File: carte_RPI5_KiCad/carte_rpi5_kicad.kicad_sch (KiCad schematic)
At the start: 0 parts

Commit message: Placement composants
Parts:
- added PS1: OKL-T_6-W12N-C, OKLT6W12NC, symbol Librairie_symbole:OKL-T_6-W12N-C
- added U1: CM5108032, CM5108032:MODULE_CM5108032, symbol Librairie_symbole:CM5108032
- added U2: BNO055, BNO055:LGA28R50P4X10_380X520X100, symbol Librairie_symbole:BNO055
- added U3: L293D, L293D:DIP880W50P254L2000H510Q16, symbol Librairie_symbole:L293D
- added U4: LPS22HB, LPS22HB:LGA10R50P2X3_200X200X80, symbol Librairie_symbole:LPS22HB
- added U5: PCA9685PW_118, PCA9685PW_118:SOP65P640X110-28N, symbol Librairie_symbole:PCA9685PW_118
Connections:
- new net: U1.SH1 (MOUNTING_PADS), U1.SH2 (MOUNTING_PADS), U1.SH3 (MOUNTING_PADS), U1.SH4 (MOUNTING_PADS)
- new net +5V(INPUT): U1.77 (+5V(INPUT)), U1.79 (+5V(INPUT)), U1.81 (+5V(INPUT)), U1.83 (+5V(INPUT)), U1.85 (+5V(INPUT)), U1.87 (+5V(INPUT))
- new net CM5_1.8V(OUTPUT): U1.88 (CM5_1.8V(OUTPUT)), U1.90 (CM5_1.8V(OUTPUT))
- new net CM5_3.3V(OUTPUT): U1.84 (CM5_3.3V(OUTPUT)), U1.86 (CM5_3.3V(OUTPUT))
- new net GND: U1.1 (GND), U1.107 (GND), U1.108 (GND), U1.113 (GND), U1.114 (GND), U1.119 (GND), U1.120 (GND), U1.125 (GND), U1.126 (GND), U1.13 (GND), U1.131 (GND), U1.132 (GND), U1.137 (GND), U1.138 (GND), U1.14 (GND), U1.144 (GND), U1.150 (GND), U1.155 (GND), U1.156 (GND), U1.161 (GND), U1.162 (GND), U1.167 (GND), U1.168 (GND), U1.173 (GND), U1.174 (GND), U1.179 (GND), U1.180 (GND), U1.185 (GND), U1.186 (GND), U1.191 (GND), U1.192 (GND), U1.197 (GND), U1.198 (GND), U1.2 (GND), U1.22 (GND), U1.23 (GND), U1.32 (GND), U1.33 (GND), U1.42 (GND), U1.43 (GND), U1.52 (GND), U1.53 (GND), U1.59 (GND), U1.60 (GND), U1.65 (GND), U1.66 (GND), U1.7 (GND), U1.71 (GND), U1.74 (GND), U1.8 (GND), U1.98 (GND), U3.12 (GND), U3.13 (GND), U3.4 (GND), U3.5 (GND), U4.8 (GND), U4.9 (GND)

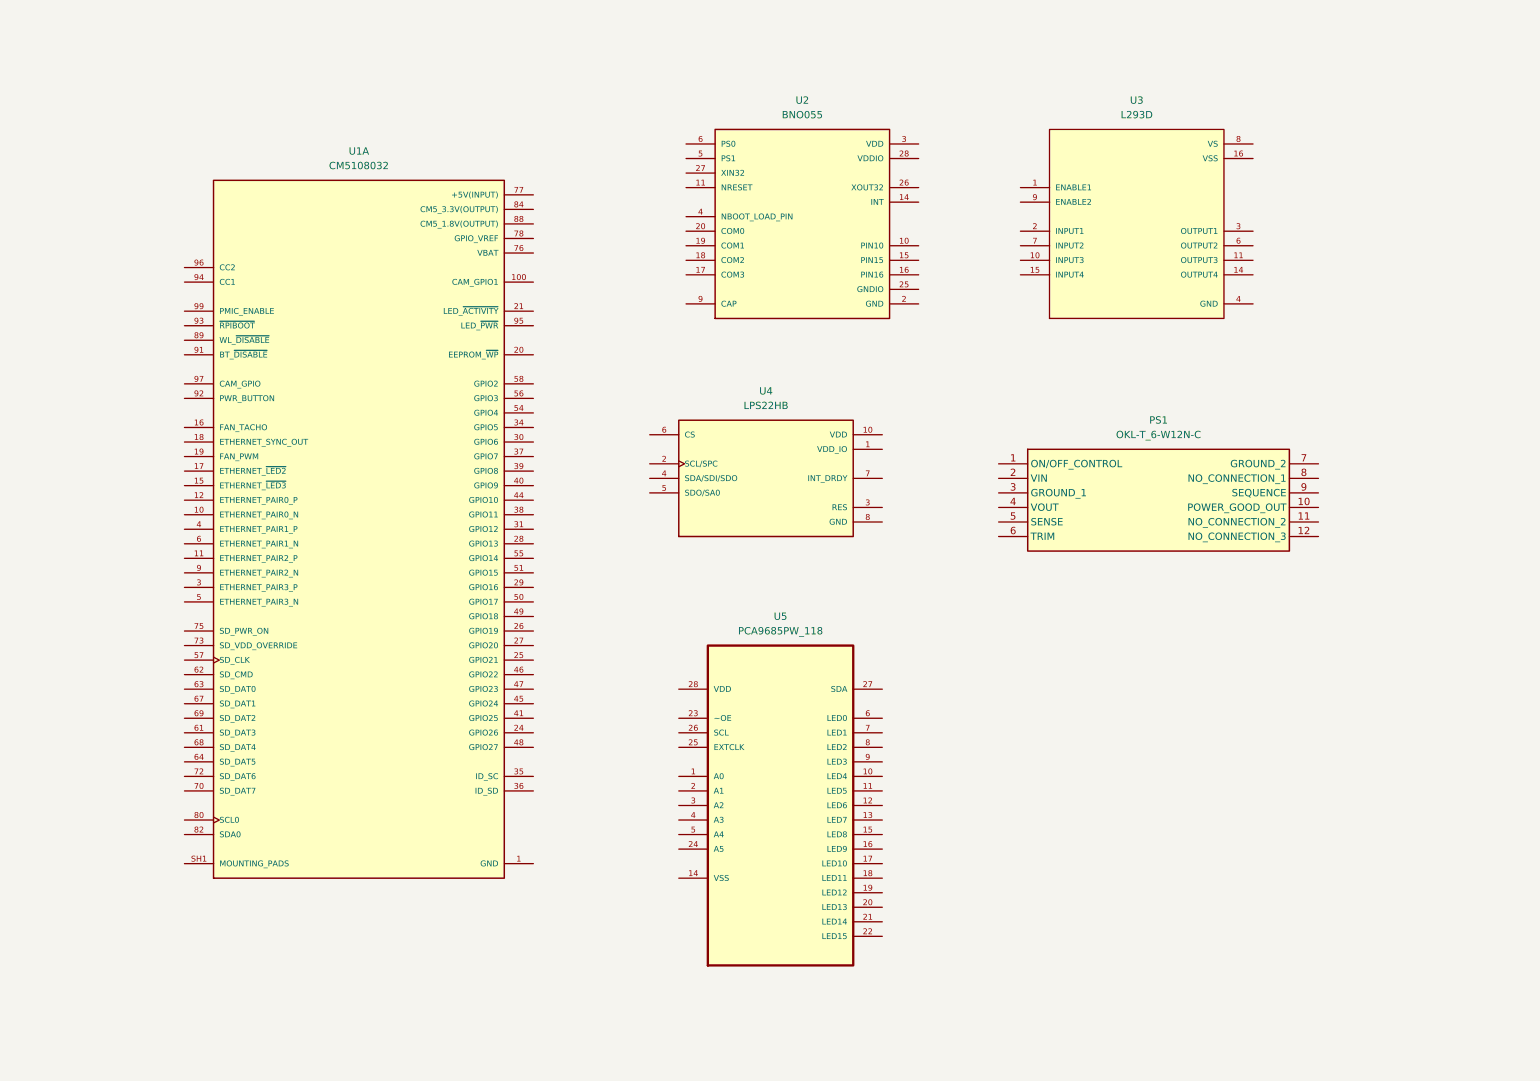
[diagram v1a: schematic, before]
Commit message: Début du schéma Kicad
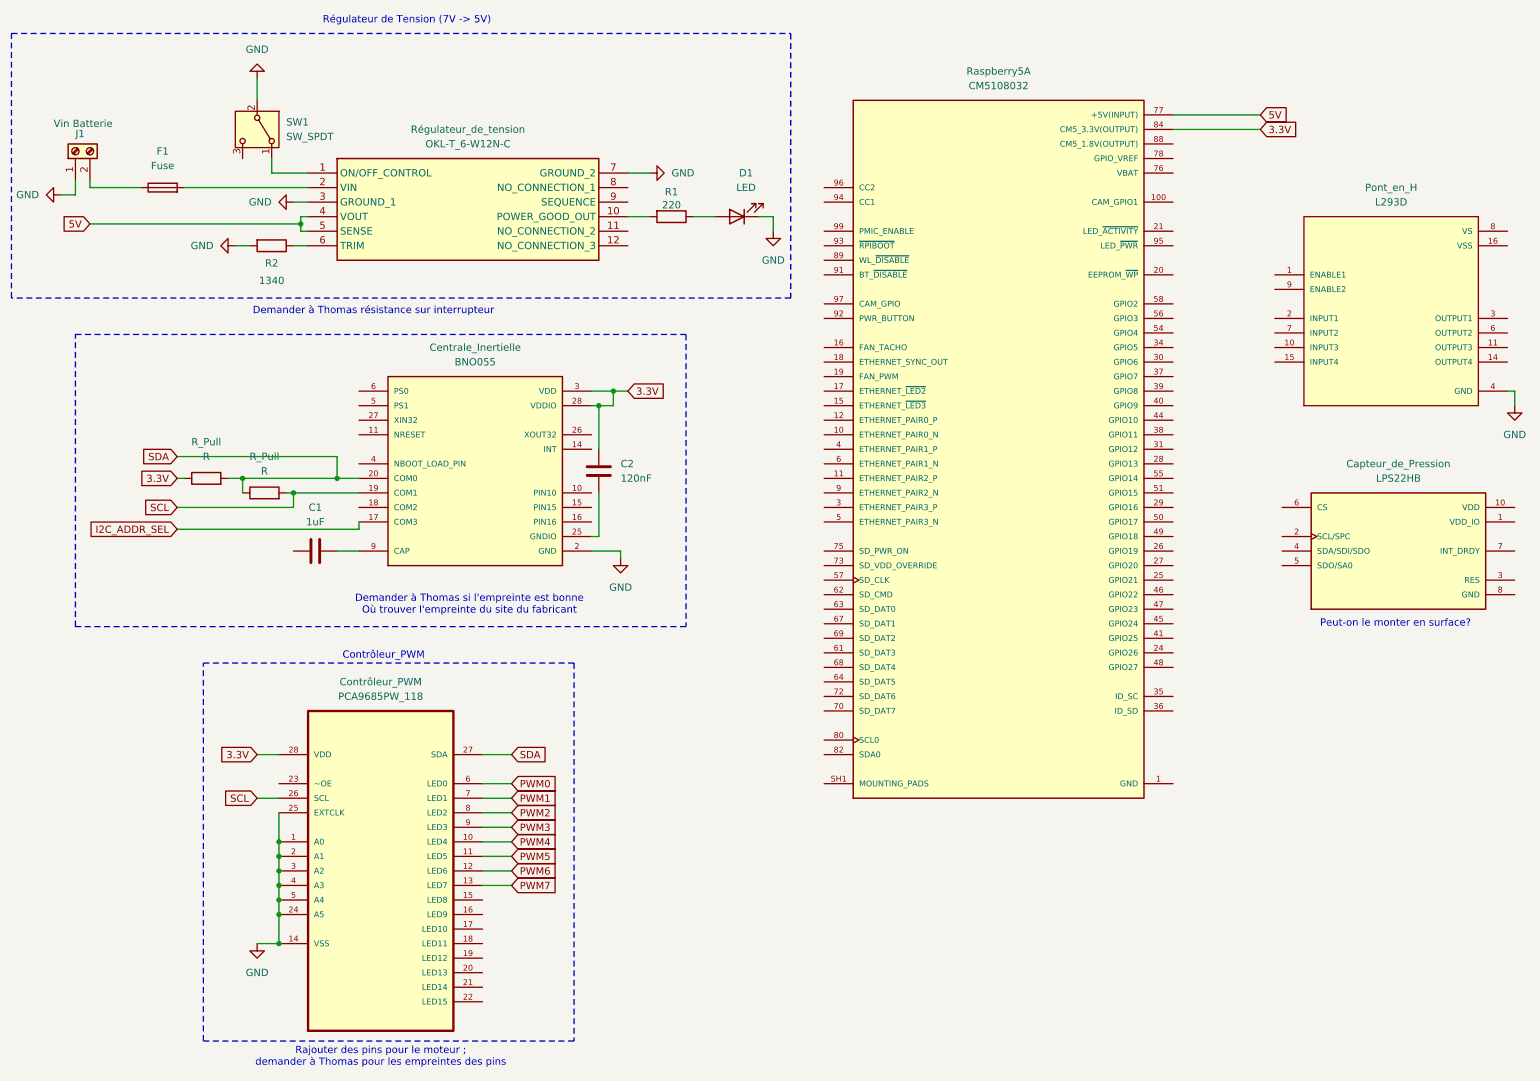
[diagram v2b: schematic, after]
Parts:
- removed PS1: OKL-T_6-W12N-C, OKLT6W12NC, symbol Librairie_symbole:OKL-T_6-W12N-C
- added C1: 1uF, symbol Device:C
- added C2: 120nF, symbol Device:C
- added D1: LED, LED_SMD:LED_0805_2012Metric, symbol Device:LED
- added F1: Fuse, Fuse:Fuse_0402_1005Metric, symbol Device:Fuse
- added J1: Vin Batterie, TerminalBlock:TerminalBlock_MaiXu_MX126-5.0-02P_1x02_P5.00mm, symbol Connector:Screw_Terminal_01x02
- added R1: 220, Resistor_SMD:R_0805_2012Metric, symbol Device:R
- added R2: 1340, Resistor_SMD:R_0805_2012Metric, symbol Device:R
- added R_Pull (x2): R, symbol Device:R
- added Régulateur_de_tension: OKL-T_6-W12N-C, Library:OKLT6W12NC, symbol OKL-T_6-W12N-C:OKL-T_6-W12N-C
- added SW1: SW_SPDT, Button_Switch_THT:SW_DIP_SPSTx01_Slide_6.7x4.1mm_W7.62mm_P2.54mm_LowProfile, symbol Switch:SW_SPDT
- renumbered U4 to Capteur_de_Pression, U2 to Centrale_Inertielle, U5 to Contrôleur_PWM, U3 to Pont_en_H, U1 to Raspberry5
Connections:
- net +5V(INPUT): now also Régulateur_de_tension.4 (VOUT), Régulateur_de_tension.5 (SENSE)
- net CM5_3.3V(OUTPUT): now also Centrale_Inertielle.28 (VDDIO), Centrale_Inertielle.3 (VDD), Contrôleur_PWM.28 (VDD), C2.2, R_Pull.1
- net GND: now also Centrale_Inertielle.2 (GND), Contrôleur_PWM.1 (A0), Contrôleur_PWM.14 (VSS), Contrôleur_PWM.2 (A1), Contrôleur_PWM.24 (A5), Contrôleur_PWM.25 (EXTCLK), Contrôleur_PWM.3 (A2), Contrôleur_PWM.4 (A3), Contrôleur_PWM.5 (A4), D1.1 (K), J1.1 (Pin_1), R2.2, Régulateur_de_tension.3 (GROUND_1), Régulateur_de_tension.7 (GROUND_2), SW1.2 (B)
- net I2C_ADDR_SEL: now reaches Centrale_Inertielle.17 (COM3)
- net SCL: now reaches Centrale_Inertielle.19 (COM1)
- net SCL: now also Contrôleur_PWM.26 (SCL), R_Pull.2
- net SDA: now reaches Centrale_Inertielle.20 (COM0)
- net SDA: now also Contrôleur_PWM.27 (SDA), R_Pull.1, R_Pull.2
- net at Centrale_Inertielle.25 (GNDIO): now also C2.1
- net at Centrale_Inertielle.9 (CAP): now also C1.2
- net PWM4: now reaches Contrôleur_PWM.10 (LED4)
- net PWM5: now reaches Contrôleur_PWM.11 (LED5)
- net PWM6: now reaches Contrôleur_PWM.12 (LED6)
- net PWM7: now reaches Contrôleur_PWM.13 (LED7)
- net PWM0: now reaches Contrôleur_PWM.6 (LED0)
- net PWM1: now reaches Contrôleur_PWM.7 (LED1)
- net PWM2: now reaches Contrôleur_PWM.8 (LED2)
- net PWM3: now reaches Contrôleur_PWM.9 (LED3)
- new net: D1.2 (A), R1.1
- new net: F1.1, J1.2 (Pin_2)
- new net: R2.1, Régulateur_de_tension.6 (TRIM)
- new net: R1.2, Régulateur_de_tension.10 (POWER_GOOD_OUT)
- new net: Régulateur_de_tension.1 (ON/OFF_CONTROL), SW1.1 (A)
- new net: F1.2, Régulateur_de_tension.2 (VIN)
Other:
- note added: "Contrôleur_PWM"
- note added: "Demander à Thomas résistance sur interrupteur"
- note added: "Demander à Thomas si l'empreinte est bonne Où trouver l'empreinte du site du fabricant"
- note added: "Peut-on le monter en surface?"
- note added: "Rajouter des pins pour le moteur ; demander à Thomas pour les empreintes des pins"
- note added: "Régulateur de Tension (7V -> 5V)"
- moved on the sheet: Capteur_de_Pression, Centrale_Inertielle, Contrôleur_PWM, Pont_en_H, Raspberry5A
